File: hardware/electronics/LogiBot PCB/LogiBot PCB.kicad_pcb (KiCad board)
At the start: 2 copper layers, 7 parts, among them U1 LM2596S-5, U2 ACS712xLCTR-20A_MRIGHT, U3 STM32G474RET6, U4 USBLC6-2SC6, U5 TJA1051T, U6 AP2112K-3.3, U7 ACS712xLCTR-20A_MLEFT

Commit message: schematic v1 finish
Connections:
- U3 pad 20: unconnected-(U3-PA6-Pad20) -> PA6
- U3 pad 21: unconnected-(U3-PA7-Pad21) -> PA7
- U3 pad 30: unconnected-(U3-PB10-Pad30) -> I2C_IMU_SCL
- U3 pad 33: unconnected-(U3-PB11-Pad33) -> I2C_IMU_SDA
- U3 pad 42: unconnected-(U3-PA8-Pad42) -> PA8
- U3 pad 43: unconnected-(U3-PA9-Pad43) -> INT
- U3 pad 44: unconnected-(U3-PA10-Pad44) -> PA10
- U3 pad 45: unconnected-(U3-PA11-Pad45) -> PA11
- U3 pad 59: unconnected-(U3-PB6-Pad59) -> I2C_IMU_SCL
- U3 pad 60: unconnected-(U3-PB7-Pad60) -> I2C_IMU_SDA

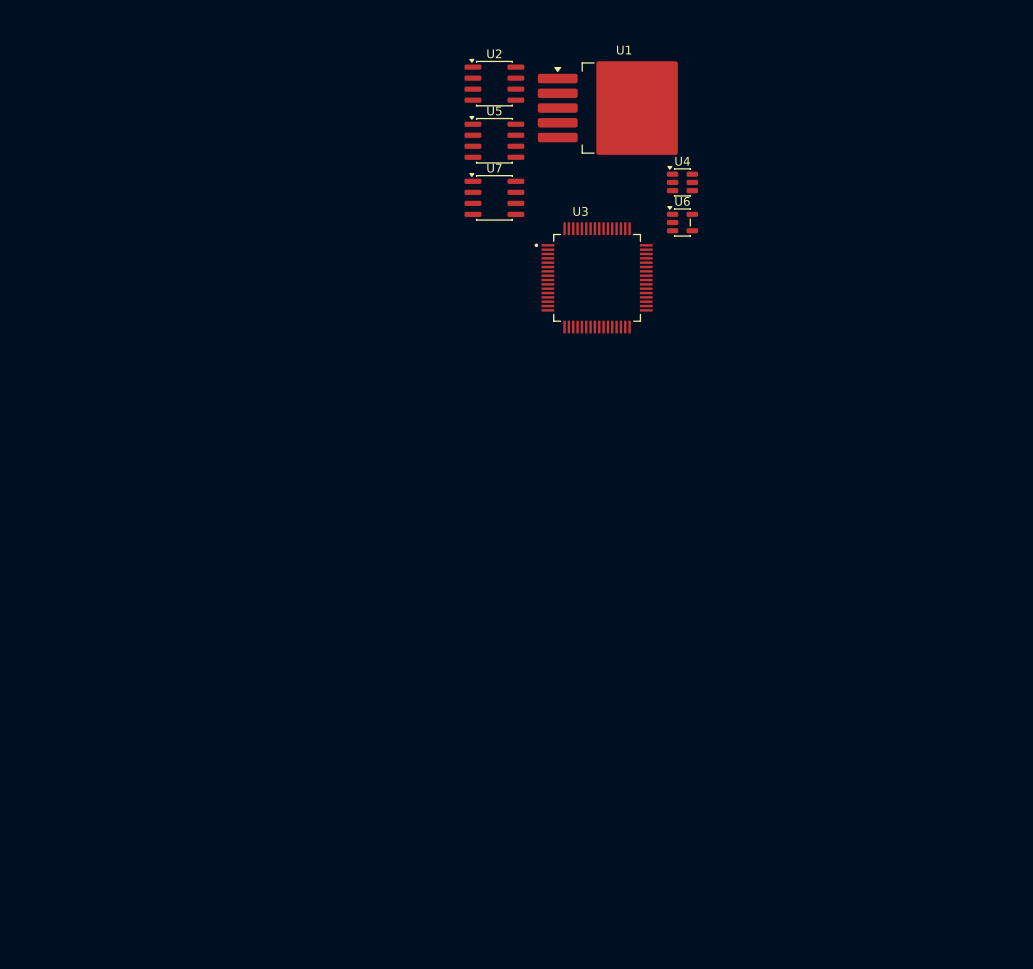
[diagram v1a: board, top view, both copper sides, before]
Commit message: pcb v1 finished
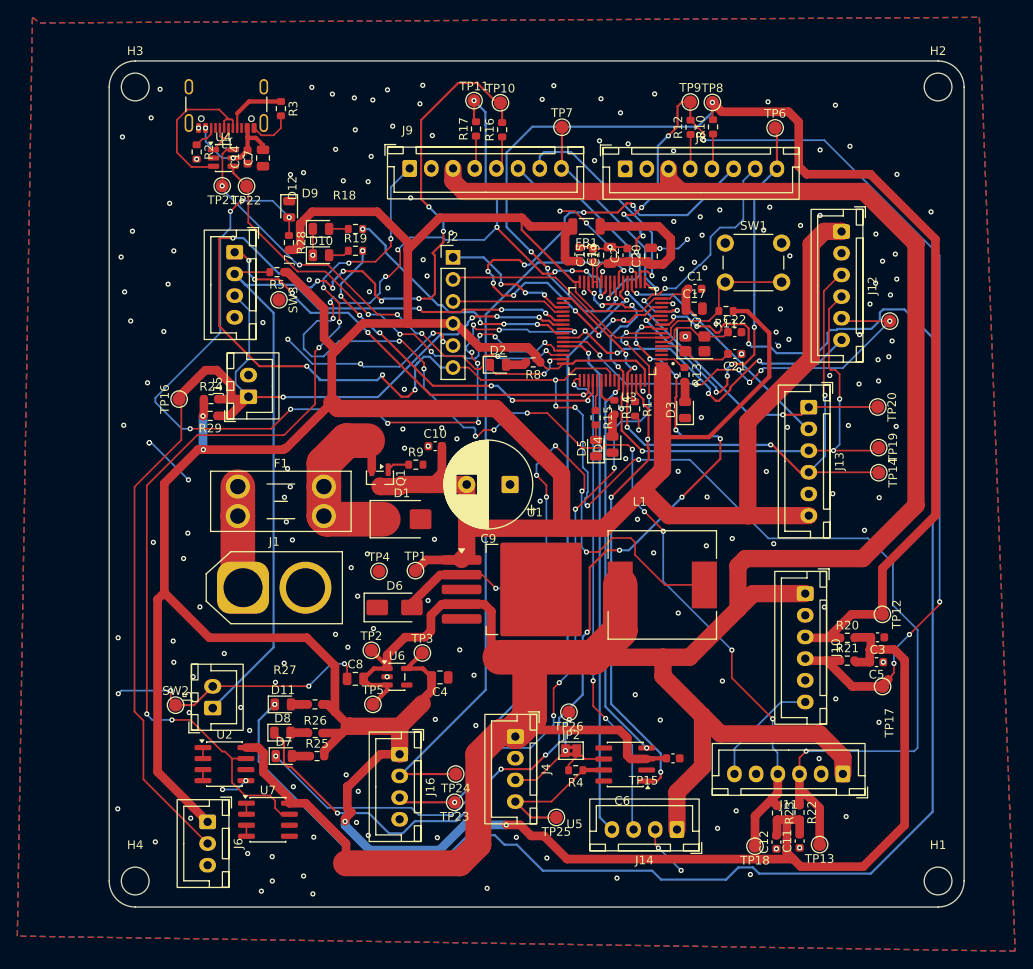
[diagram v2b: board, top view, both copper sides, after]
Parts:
- added C1: 100nF, Capacitor_SMD:C_0603_1608Metric, F.Cu at (117.9, 94.7)
- added C10: 100nF, Capacitor_SMD:C_0603_1608Metric, F.Cu at (88.0, 112.9)
- added C11: 100pF, Capacitor_SMD:C_0603_1608Metric, F.Cu at (130.0, 158.4)
- added C12: 100pF, Capacitor_SMD:C_0603_1608Metric, F.Cu at (127.3, 158.5)
- added C13: 100nF, Capacitor_SMD:C_0603_1608Metric, F.Cu at (104.6, 90.7)
- added C14: 100nF, Capacitor_SMD:C_0603_1608Metric, F.Cu at (66.3, 79.5)
- added C15: 100nF, Capacitor_SMD:C_0603_1608Metric, F.Cu at (106.2, 90.9)
- added C17: 4.7uF, Capacitor_SMD:C_0805_2012Metric, F.Cu at (117.8, 97.0)
- added C19: 1uF, Capacitor_SMD:C_0805_2012Metric, F.Cu at (108.1, 90.9)
- added C2: 100nF, Capacitor_SMD:C_0603_1608Metric, F.Cu at (110.1, 90.8)
- added C20: 1uF, Capacitor_SMD:C_0805_2012Metric, F.Cu at (112.8, 91.0)
- added C21: 22pF, Capacitor_SMD:C_0603_1608Metric, F.Cu at (122.5, 102.2)
- added C22: 22pF, Capacitor_SMD:C_0603_1608Metric, F.Cu at (122.5, 99.7)
- added C3: 100pF, Capacitor_SMD:C_0603_1608Metric, F.Cu at (139.0, 134.9)
- added C4: 10uF, Capacitor_SMD:C_0805_2012Metric, F.Cu at (88.5, 139.5)
- added C5: 100pF, Capacitor_SMD:C_0603_1608Metric, F.Cu at (138.9, 137.8)
- added C6: 100nF, Capacitor_SMD:C_0603_1608Metric, F.Cu at (115.4, 148.9)
- added C7: 10uF, Capacitor_SMD:C_0805_2012Metric, F.Cu at (68.1, 79.6)
- added C8: 10uF, Capacitor_SMD:C_0805_2012Metric, F.Cu at (78.8, 139.7)
- added C9: 100uF, Capacitor_THT:CP_Radial_D10.0mm_P5.00mm, F.Cu at (96.6, 117.3)
- added D1: SMBJ33A, Diode_SMD:D_SMB, F.Cu at (84.1, 121.3)
- added D10: LED_STATUS L, LED_SMD:LED_0805_2012Metric, F.Cu at (74.8, 90.8)
- added D11: LED_BLUE_UART, LED_SMD:LED_0805_2012Metric, F.Cu at (70.4, 142.6)
- added D12: Safety LED, LED_SMD:LED_0805_2012Metric, F.Cu at (71.1, 85.6)
- added D2: LED_POWER, LED_SMD:LED_0805_2012Metric, F.Cu at (95.2, 103.5)
- added D3: LED_RUN, LED_SMD:LED_0805_2012Metric, F.Cu at (116.8, 108.7)
- added D4: LED_ERROR, LED_SMD:LED_0805_2012Metric, F.Cu at (108.4, 112.7)
- added D5: LED_COMM, LED_SMD:LED_0805_2012Metric, F.Cu at (106.5, 113.1)
- added D6: SS34, Diode_SMD:D_SMA, F.Cu at (83.3, 131.5)
- added D7: LED_GREEN_USB, LED_SMD:LED_0805_2012Metric, F.Cu at (70.5, 148.6)
- added D8: LED_YELLOW_CAN, LED_SMD:LED_0805_2012Metric, F.Cu at (70.4, 145.9)
- added D9: LED_STATUS R, LED_SMD:LED_0805_2012Metric, F.Cu at (74.8, 87.8)
- added F1: 10A, Fuse:Fuseholder_Blade_Mini_Keystone_3568, F.Cu at (65.2, 117.5)
- added FB1: FerriteBead, Inductor_SMD:L_1206_3216Metric, F.Cu at (105.4, 87.5)
- added H1: MountingHole, MountingHole:MountingHole_3.2mm_M3, F.Cu at (145.9, 163.0)
- added H2: MountingHole, MountingHole:MountingHole_3.2mm_M3, F.Cu at (145.9, 71.5)
- added H3: MountingHole, MountingHole:MountingHole_3.2mm_M3, F.Cu at (53.4, 71.5)
- added H4: MountingHole, MountingHole:MountingHole_3.2mm_M3, F.Cu at (53.4, 163.0)
- added J1: XT60, Connector_AMASS:AMASS_XT60-M_1x02_P7.20mm_Vertical, F.Cu at (65.8, 129.2)
- added J10: ENCODER_LEFT, Connector_JST:JST_XH_B6B-XH-A_1x06_P2.50mm_Vertical, F.Cu at (130.6, 129.9)
- added J11: ENCODER_RIGHT, Connector_JST:JST_XH_B6B-XH-A_1x06_P2.50mm_Vertical, F.Cu at (135.0, 150.7)
- added J12: J_IMU, Connector_JST:JST_XH_B6B-XH-A_1x06_P2.50mm_Vertical, F.Cu at (134.8, 88.1)
- added J13: VL53L0X, Connector_JST:JST_XH_B6B-XH-A_1x06_P2.50mm_Vertical, F.Cu at (131.0, 108.4)
- added J14: Ultrasonic Header, Connector_JST:JST_XH_B4B-XH-A_1x04_P2.50mm_Vertical, F.Cu at (115.8, 157.1)
- added J15: Bumper Switch, Connector_JST:JST_XH_B2B-XH-A_1x02_P2.50mm_Vertical, F.Cu at (66.4, 107.2)
- added J16: UART STM32 ↔ ORANGE PI, Connector_JST:JST_XH_B4B-XH-A_1x04_P2.50mm_Vertical, F.Cu at (83.9, 148.4)
- added J2: SWD Debug, Connector_PinHeader_2.54mm:PinHeader_1x06_P2.54mm_Vertical, F.Cu at (90.0, 91.1)
- added J3: USB_C_Receptacle_USB2.0_16P, Connector_USB:USB_C_Receptacle_GCT_USB4105-xx-A_16P_TopMnt_Horizontal, F.Cu at (63.9, 72.5)
- added J4: Konektor CAN, Connector_JST:JST_XH_B4B-XH-A_1x04_P2.50mm_Vertical, F.Cu at (97.2, 146.4)
- added J5: Emergency Stop Connector, Connector_JST:JST_XH_B2B-XH-A_1x02_P2.50mm_Vertical, F.Cu at (62.3, 143.1)
- added J6: Bumper Switch Connector, Connector_JST:JST_XH_B3B-XH-A_1x03_P2.50mm_Vertical, F.Cu at (61.7, 156.2)
- added J7: Safety Header, Connector_JST:JST_XH_B4B-XH-A_1x04_P2.50mm_Vertical, F.Cu at (64.8, 90.5)
- added J8: MotorDriver_Left, Connector_JST:JST_XH_B8B-XH-A_1x08_P2.50mm_Vertical, F.Cu at (109.9, 80.9)
- added J9: MotorDriver_Right, Connector_JST:JST_XH_B8B-XH-A_1x08_P2.50mm_Vertical, F.Cu at (85.0, 80.8)
- added JP2: Jumper_2_Open, Jumper:SolderJumper-2_P1.3mm_Bridged2Bar_Pad1.0x1.5mm, F.Cu at (103.6, 148.0)
- added L1: 33uH, INDP125125X600N:INDP125125X600N, F.Cu at (114.2, 128.9)
- added Q1: Q_PMOS_GSD, Package_TO_SOT_SMD:SOT-23, F.Cu at (81.6, 116.5)
- added R1: 10K, Resistor_SMD:R_0603_1608Metric, F.Cu at (111.0, 108.6)
- added R10: 4.7K, Resistor_SMD:R_0603_1608Metric, F.Cu at (120.0, 76.0)
- added R11: 10K, Resistor_SMD:R_0603_1608Metric, F.Cu at (121.5, 97.3)
- added R12: 4.7K, Resistor_SMD:R_0603_1608Metric, F.Cu at (117.4, 76.1)
- added R13: 330, Resistor_SMD:R_0603_1608Metric, F.Cu at (116.7, 104.6)
- added R14: 330, Resistor_SMD:R_0603_1608Metric, F.Cu at (108.6, 108.4)
- added R15: 330, Resistor_SMD:R_0603_1608Metric, F.Cu at (106.5, 109.6)
- added R16: 4.7K, Resistor_SMD:R_0603_1608Metric, F.Cu at (95.7, 76.4)
- added R17: 4.7K, Resistor_SMD:R_0603_1608Metric, F.Cu at (92.7, 76.3)
- added R18: 330, Resistor_SMD:R_0603_1608Metric, F.Cu at (78.8, 87.8)
- added R19: 330, Resistor_SMD:R_0603_1608Metric, F.Cu at (78.8, 90.3)
- added R2: 5.1K, Resistor_SMD:R_0603_1608Metric, F.Cu at (60.5, 78.9)
- added R20: 10K, Resistor_SMD:R_0603_1608Metric, F.Cu at (135.5, 135.0)
- added R21: 10K, Resistor_SMD:R_0603_1608Metric, F.Cu at (135.5, 137.6)
- added R22: 10K, Resistor_SMD:R_0603_1608Metric, F.Cu at (130.0, 155.1)
- added R23: 10K, Resistor_SMD:R_0603_1608Metric, F.Cu at (127.4, 155.2)
- added R24: 10K, Resistor_SMD:R_0603_1608Metric, F.Cu at (62.1, 107.4)
- added R25: 330, Resistor_SMD:R_0603_1608Metric, F.Cu at (74.3, 148.6)
- added R26: 330, Resistor_SMD:R_0603_1608Metric, F.Cu at (74.1, 145.9)
- added R27: 330, Resistor_SMD:R_0603_1608Metric, F.Cu at (74.1, 142.6)
- added R28: 330, Resistor_SMD:R_0603_1608Metric, F.Cu at (71.1, 89.4)
- added R29: 10k, Resistor_SMD:R_0603_1608Metric, F.Cu at (62.0, 109.4)
- added R3: 5.1K, Resistor_SMD:R_0603_1608Metric, F.Cu at (70.2, 74.0)
- added R4: 120, Resistor_SMD:R_0603_1608Metric, F.Cu at (104.2, 150.2)
- added R5: 10k, Resistor_SMD:R_0603_1608Metric, F.Cu at (69.7, 92.8)
- added R8: 330, Resistor_SMD:R_0603_1608Metric, F.Cu at (99.3, 103.2)
- added R9: 100K, Resistor_SMD:R_0603_1608Metric, F.Cu at (85.7, 115.0)
- added SW1: BUTTON_RST, Button_Switch_THT:SW_PUSH_6mm, F.Cu at (121.4, 89.5)
- added SW2: E-Stop Switch, TestPoint:TestPoint_Pad_D1.5mm, F.Cu at (58.0, 142.7)
- added SW3: Bumper Switch, TestPoint:TestPoint_Pad_D1.5mm, F.Cu at (69.9, 96.0)
- added TP1: TP_VBAT, TestPoint:TestPoint_Pad_D1.5mm, F.Cu at (85.7, 127.2)
- added TP10: TP_ENC_R_A, TestPoint:TestPoint_Pad_D1.5mm, F.Cu at (95.5, 73.3)
- added TP11: TP_ENC_R_B, TestPoint:TestPoint_Pad_D1.5mm, F.Cu at (92.4, 73.0)
- added TP12: ENC_L_A, TestPoint:TestPoint_Pad_D1.5mm, F.Cu at (139.5, 132.3)
- added TP13: ENC_R_A, TestPoint:TestPoint_Pad_D1.5mm, F.Cu at (132.3, 158.8)
- added TP14: SDA, TestPoint:TestPoint_Pad_D1.5mm, F.Cu at (139.1, 115.9)
- added TP15: IMU INT, TestPoint:TestPoint_Pad_D1.5mm, F.Cu at (140.4, 98.5)
- added TP16: BUMPER, TestPoint:TestPoint_Pad_D1.5mm, F.Cu at (58.4, 107.4)
- added TP17: ENC_L_B, TestPoint:TestPoint_Pad_D1.5mm, F.Cu at (139.6, 140.6)
- added TP18: ENC_R_B, TestPoint:TestPoint_Pad_D1.5mm, F.Cu at (124.8, 159.0)
- added TP19: SCL, TestPoint:TestPoint_Pad_D1.5mm, F.Cu at (139.1, 113.0)
- added TP2: TP_5V, TestPoint:TestPoint_Pad_D1.5mm, F.Cu at (80.6, 136.4)
- added TP20: TP8 VL53_INT, TestPoint:TestPoint_Pad_D1.5mm, F.Cu at (139.0, 108.3)
- added TP21: USB_DP, TestPoint:TestPoint_Pad_D1.5mm, F.Cu at (63.4, 82.8)
- added TP22: USB_DM, TestPoint:TestPoint_Pad_D1.5mm, F.Cu at (66.2, 82.9)
- added TP23: UART_TX, TestPoint:TestPoint_Pad_D1.5mm, F.Cu at (90.2, 153.9)
- added TP24: UART_RX, TestPoint:TestPoint_Pad_D1.5mm, F.Cu at (90.3, 150.7)
- added TP25: CANH, TestPoint:TestPoint_Pad_D1.5mm, F.Cu at (101.9, 155.7)
- added TP26: CANL, TestPoint:TestPoint_Pad_D1.5mm, F.Cu at (103.4, 143.5)
- added TP3: TP_3V3, TestPoint:TestPoint_Pad_D1.5mm, F.Cu at (86.5, 136.7)
- added TP4: TP_GND, TestPoint:TestPoint_Pad_D1.5mm, F.Cu at (81.5, 127.3)
- added TP5: TP_5V, TestPoint:TestPoint_Pad_D1.5mm, F.Cu at (80.8, 142.6)
- added TP6: TP_PWM_L, TestPoint:TestPoint_Pad_D1.5mm, F.Cu at (127.2, 76.2)
- added TP7: TP_PWM_R, TestPoint:TestPoint_Pad_D1.5mm, F.Cu at (102.6, 76.1)
- added TP8: TP_ENC_L_A, TestPoint:TestPoint_Pad_D1.5mm, F.Cu at (119.9, 73.2)
- added TP9: TP_ENC_L_B, TestPoint:TestPoint_Pad_D1.5mm, F.Cu at (117.4, 73.2)
- added Y2: 8MHz, Crystal:Crystal_SMD_3225-4Pin_3.2x2.5mm, F.Cu at (117.9, 101.1)
- moved U2 84.4 mm to (63.7, 149.5)
- moved U7 76.3 mm to (68.7, 155.9)
- moved U5 73.5 mm to (109.9, 149.6), turned to 180 degrees
- moved U6 61.9 mm to (83.6, 139.5)
- moved U1 56.6 mm to (98.7, 129.4)
- moved U4 53.0 mm to (63.5, 79.6)
- moved U3 6.39 mm to (108.4, 99.6), turned to 180 degrees
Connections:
- U3 pad 10: unconnected-(U3-PC2-Pad10) -> PC2
- U3 pad 22: unconnected-(U3-PC4-Pad22) -> PC4
- U3 pad 23: unconnected-(U3-PC5-Pad23) -> PC5
- U3 pad 28: 24V_MOTOR -> VDDA
- U3 pad 29: 24V_MOTOR -> VDDA
- U3 pad 38: unconnected-(U3-PC6-Pad38) -> ESTOP
- U3 pad 39: unconnected-(U3-PC7-Pad39) -> BUMPER
- U3 pad 40: unconnected-(U3-PC8-Pad40) -> SAFETY_LED_GPIO
- U3 pad 46: unconnected-(U3-PA12-Pad46) -> PA12
- U3 pad 49: unconnected-(U3-PA13-Pad49) -> PA13
- U3 pad 51: unconnected-(U3-PA15-Pad51) -> SAFETY_OUT
- U3 pad 58: unconnected-(U3-PB5-Pad58) -> CAN1_RX
- U3 pad 62: unconnected-(U3-PB9-Pad62) -> CAN1_TX
- U3 pad 8: unconnected-(U3-PC0-Pad8) -> PC0
- U3 pad 9: unconnected-(U3-PC1-Pad9) -> PC1
- U4 pad 1: unconnected-(U4-I/O1-Pad1) -> Net-(J3-D+-PadA6)
- U4 pad 2: unconnected-(U4-GND-Pad2) -> BAT-
- U4 pad 3: unconnected-(U4-I/O2-Pad3) -> Net-(J3-D--PadA7)
- U4 pad 4: unconnected-(U4-I/O2-Pad4) -> PA11
- U4 pad 5: unconnected-(U4-VBUS-Pad5) -> +5V USB
- U4 pad 6: unconnected-(U4-I/O1-Pad6) -> PA12
- U5 pad 1: unconnected-(U5-TXD-Pad1) -> CAN1_TX
- U5 pad 2: unconnected-(U5-GND-Pad2) -> BAT-
- U5 pad 3: unconnected-(U5-VCC-Pad3) -> 5V_MAIN
- U5 pad 4: unconnected-(U5-RXD-Pad4) -> CAN1_RX
- U5 pad 6: unconnected-(U5-CANL-Pad6) -> Net-(JP2-B)
- U5 pad 7: unconnected-(U5-CANH-Pad7) -> CANH
- U5 pad 8: unconnected-(U5-S-Pad8) -> BAT-
- U6 pad 5: 3V3 -> 24V_MOTOR
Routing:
- net 24V_MOTOR: track 0.00 -> 591.5 mm, vias 0 -> 4
- net 5V_MAIN: track 0.00 -> 326.9 mm
- net ENC_R_A: track 0.00 -> 242.7 mm, vias 0 -> 17
- net PC2: track 0.00 -> 192.0 mm, vias 0 -> 4
- net ENC_R_B: track 0.00 -> 174.5 mm, vias 0 -> 20
- net ENC_L_A: track 0.00 -> 149.7 mm, vias 0 -> 4
- net ENC_L_B: track 0.00 -> 135.1 mm, vias 0 -> 10
- net BUMPER: track 0.00 -> 129.4 mm, vias 0 -> 4
- net BAT-: track 0.00 -> 113.9 mm, vias 0 -> 205
- net PC1: track 0.00 -> 110.8 mm, vias 0 -> 12
- net CURRENT_R: track 0.00 -> 110.2 mm, vias 0 -> 7
- net SAFETY_LED_GPIO: track 0.00 -> 102.1 mm, vias 0 -> 12
- net ESTOP: track 0.00 -> 99.3 mm, vias 0 -> 3
- net PC0: track 0.00 -> 98.3 mm, vias 0 -> 8
- net PC5: track 0.00 -> 84.5 mm, vias 0 -> 1
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- added copper zone on B.Cu, net BAT-
- added copper zone on F.Cu, net BAT-
- added copper zone on In1.Cu, net BAT-
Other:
- board outline added: 98.6 x 97.6 mm
- copper layers 2 -> 4
